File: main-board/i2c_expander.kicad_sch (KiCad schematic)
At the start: 2 parts, among them U21 TCA9548ARGER, U22 TCA9548ARGER

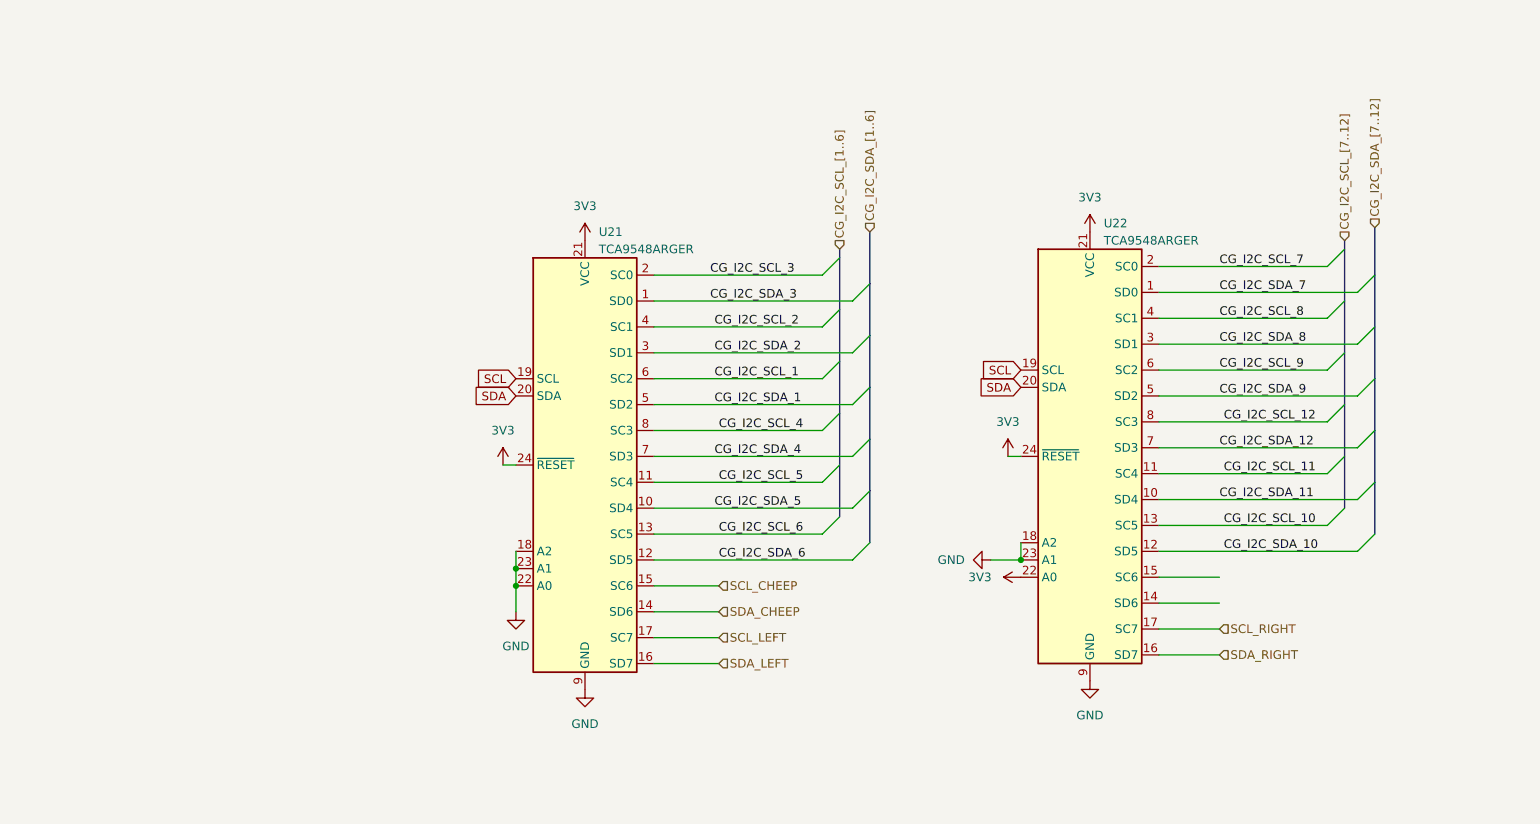
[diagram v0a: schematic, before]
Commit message: PCB update
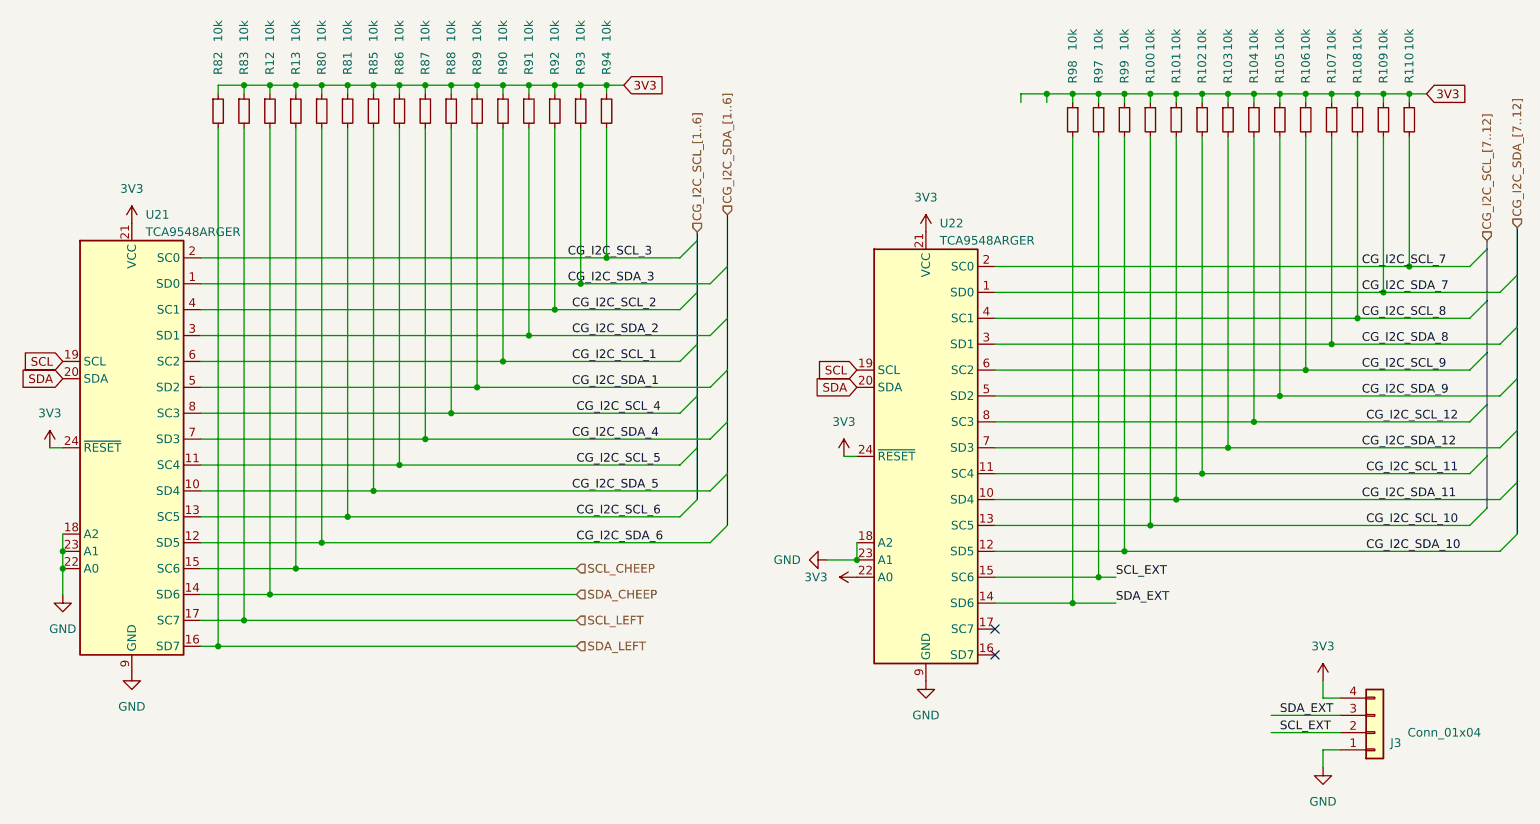
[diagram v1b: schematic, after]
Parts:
- added J3: Conn_01x04, Connector_PinSocket_2.54mm:PinSocket_1x04_P2.54mm_Vertical, symbol Connector_Generic:Conn_01x04
- added R100, R101, R102, R103, R104, R105, R106, R107, R108, R109, R110, R12, R13, R80, R81, R82, R83, R85, R86, R87, R88, R89, R90, R91, R92, R93, R94, R97, R98, R99: 10k, Resistor_SMD:R_0603_1608Metric, symbol Device:R_Small
- U21, U22: LCSC (none) -> C555456
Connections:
- net 3V3: now also J3.4 (Pin_4), R100.1, R101.1, R102.1, R103.1, R104.1, R105.1, R106.1, R107.1, R108.1, R109.1, R110.1, R12.1, R13.1, R80.1, R81.1, R82.1, R83.1, R85.1, R86.1, R87.1, R88.1, R89.1, R90.1, R91.1, R92.1, R93.1, R94.1, R97.1, R98.1, R99.1
- net CG_I2C_SCL_1: now also R90.2
- net CG_I2C_SCL_10: now also R100.2
- net CG_I2C_SCL_11: now also R102.2
- net CG_I2C_SCL_12: now also R104.2
- net CG_I2C_SCL_2: now also R92.2
- net CG_I2C_SCL_3: now also R94.2
- net CG_I2C_SCL_4: now also R88.2
- net CG_I2C_SCL_5: now also R86.2
- net CG_I2C_SCL_6: now also R81.2
- net CG_I2C_SCL_7: now also R110.2
- net CG_I2C_SCL_8: now also R108.2
- net CG_I2C_SCL_9: now also R106.2
- net CG_I2C_SDA_1: now also R89.2
- net CG_I2C_SDA_10: now also R99.2
- net CG_I2C_SDA_11: now also R101.2
- net CG_I2C_SDA_12: now also R103.2
- net CG_I2C_SDA_2: now also R91.2
- net CG_I2C_SDA_3: now also R93.2
- net CG_I2C_SDA_4: now also R87.2
- net CG_I2C_SDA_5: now also R85.2
- net CG_I2C_SDA_6: now also R80.2
- net CG_I2C_SDA_7: now also R109.2
- net CG_I2C_SDA_8: now also R107.2
- net CG_I2C_SDA_9: now also R105.2
- net GND: now also J3.1 (Pin_1)
- net SCL_CHEEP: now also R13.2
- net SCL_LEFT: now also R83.2
- net SDA_CHEEP: now also R12.2
- net SDA_LEFT: now also R82.2
- net SDA_EXT: now reaches U22.14 (SD6)
- net SDA_EXT: now also J3.3 (Pin_3), R98.2
- net SCL_EXT: now reaches U22.15 (SC6)
- net SCL_EXT: now also J3.2 (Pin_2), R97.2
- net SCL_RIGHT: no longer names the net of U22.17 (SC7)
- net SDA_RIGHT: no longer names the net of U22.16 (SD7)
- no-connect marks 0 -> 2
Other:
- moved on the sheet: U21, U22
